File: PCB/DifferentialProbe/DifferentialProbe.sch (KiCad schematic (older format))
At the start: 33 parts, among them U1 IFNU411, U2 HFA3046BZ

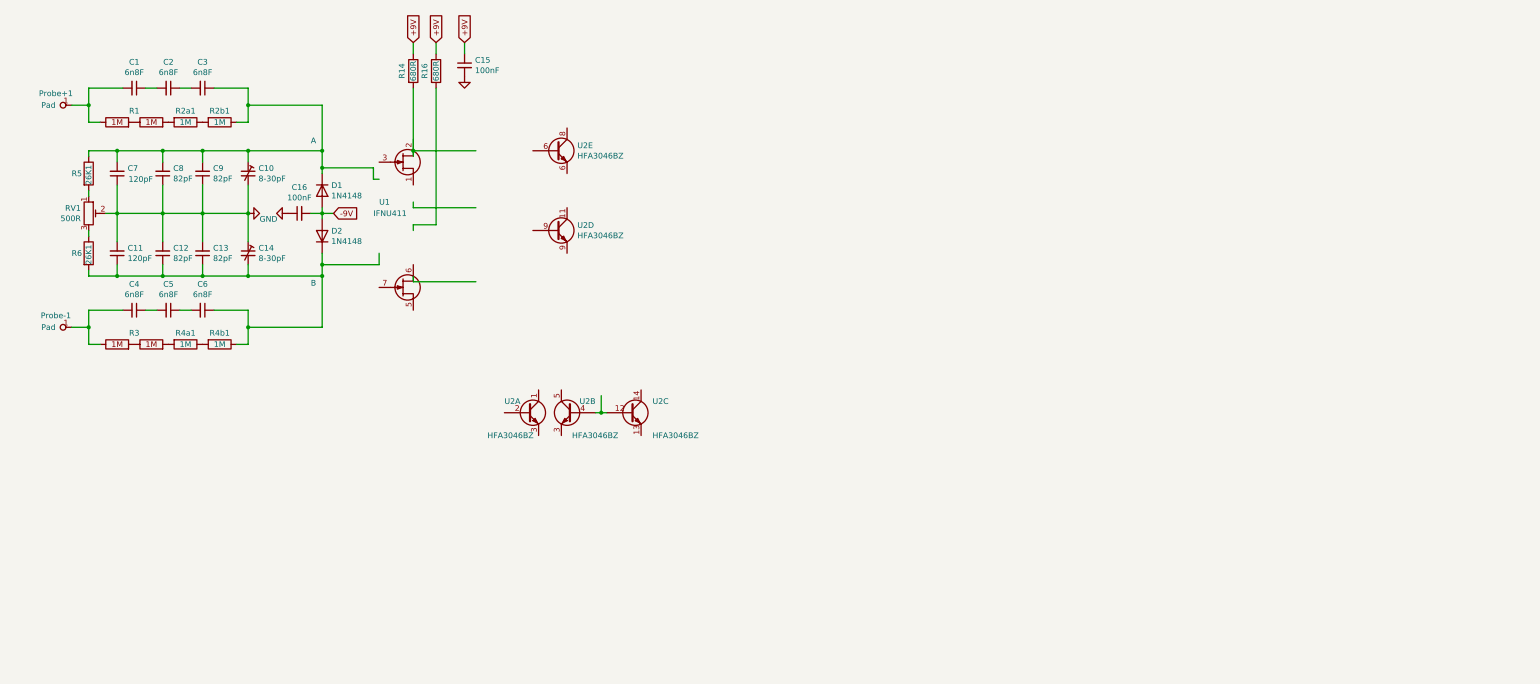
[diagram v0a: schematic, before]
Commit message: 1st design finished
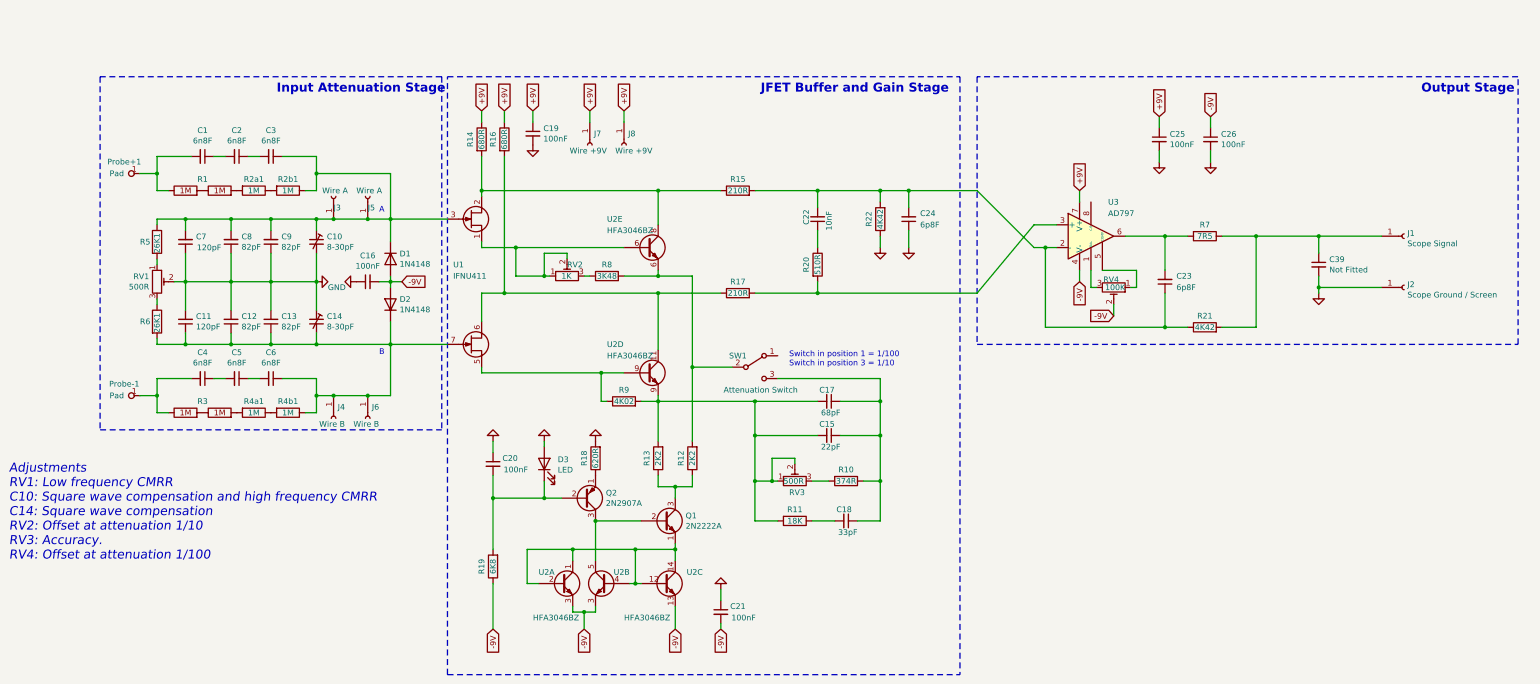
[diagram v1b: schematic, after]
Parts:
- added C15: 22pF, Capacitor_THT:C_Disc_D3.0mm_W1.6mm_P2.50mm, symbol Device:C_Small
- added C17: 68pF, Capacitor_THT:C_Disc_D3.0mm_W1.6mm_P2.50mm, symbol Device:C_Small
- added C18: 33pF, Capacitor_THT:C_Disc_D3.0mm_W1.6mm_P2.50mm, symbol Device:C_Small
- added C20, C21, C25, C26: 100nF, Capacitor_THT:C_Disc_D4.3mm_W1.9mm_P5.00mm, symbol Device:C_Small
- added C22: 10nF, Capacitor_THT:C_Disc_D3.0mm_W1.6mm_P2.50mm, symbol Device:C_Small
- added C23, C24: 6p8F, Capacitor_THT:C_Disc_D3.0mm_W1.6mm_P2.50mm, symbol Device:C_Small
- added C39: Not Fitted, Capacitor_THT:C_Disc_D4.3mm_W1.9mm_P5.00mm, symbol Device:C_Small
- added D3: LED, LED_THT:LED_D3.0mm, symbol Device:LED
- added J1: Scope Signal, Connector_Wire:SolderWire-2.5sqmm_1x01_D2.4mm_OD4.4mm, symbol Connector:Conn_01x01_Female
- added J2: Scope Ground / Screen, Connector_Wire:SolderWire-2.5sqmm_1x01_D2.4mm_OD4.4mm, symbol Connector:Conn_01x01_Female
- added J3, J5: Wire A, BVKSound:Wire_Hole, symbol BVKSound:Wire
- added J4, J6: Wire B, BVKSound:Wire_Hole, symbol BVKSound:Wire
- added J7, J8: Wire +9V, BVKSound:Wire_Hole, symbol BVKSound:Wire
- added Q1: 2N2222A, Package_TO_SOT_THT:TO-18-3, symbol Device:Q_NPN_EBC
- added Q2: 2N2907A, Package_TO_SOT_THT:TO-18-3, symbol Device:Q_PNP_EBC
- added R10: 374R, Resistor_THT:R_Axial_DIN0207_L6.3mm_D2.5mm_P10.16mm_Horizontal, symbol Device:R
- added R11: 18K, Resistor_THT:R_Axial_DIN0204_L3.6mm_D1.6mm_P7.62mm_Horizontal, symbol Device:R
- added R12, R13: 2K2, Resistor_THT:R_Axial_DIN0207_L6.3mm_D2.5mm_P10.16mm_Horizontal, symbol Device:R
- added R15: 210R, Resistor_THT:R_Axial_DIN0207_L6.3mm_D2.5mm_P10.16mm_Horizontal, symbol Device:R
- added R17: 210R, Resistor_THT:R_Axial_DIN0207_L6.3mm_D2.5mm_P2.54mm_Vertical, symbol Device:R
- added R18: 620R, Resistor_THT:R_Axial_DIN0207_L6.3mm_D2.5mm_P2.54mm_Vertical, symbol Device:R
- added R19: 6K8, Resistor_THT:R_Axial_DIN0207_L6.3mm_D2.5mm_P10.16mm_Horizontal, symbol Device:R
- added R20: 510R, Resistor_THT:R_Axial_DIN0204_L3.6mm_D1.6mm_P7.62mm_Horizontal, symbol Device:R
- added R21, R22: 4K42, Resistor_THT:R_Axial_DIN0207_L6.3mm_D2.5mm_P10.16mm_Horizontal, symbol Device:R
- added R7: 7R5, Resistor_THT:R_Axial_DIN0204_L3.6mm_D1.6mm_P7.62mm_Horizontal, symbol Device:R
- added R8: 3K48, Resistor_THT:R_Axial_DIN0207_L6.3mm_D2.5mm_P10.16mm_Horizontal, symbol Device:R
- added R9: 4K02, Resistor_THT:R_Axial_DIN0207_L6.3mm_D2.5mm_P10.16mm_Horizontal, symbol Device:R
- added RV2: 1K, BVKSound:67WR10KLF, symbol Device:R_POT_TRIM
- added RV3: 500R, BVKSound:3362P_1, symbol Device:R_POT_TRIM
- added RV4: 100K, BVKSound:64W_1, symbol Device:R_POT_TRIM
- added SW1: Attenuation Switch, BVKSound:SSSF011700, symbol Switch:SW_SPDT
- added U3: AD797, Package_DIP:DIP-8_W7.62mm, symbol Amplifier_Operational:AD797
- R16: footprint Resistor_THT:R_Axial_DIN0204_L3.6mm_D1.6mm_P2.54mm_Vertical -> Resistor_THT:R_Axial_DIN0207_L6.3mm_D2.5mm_P2.54mm_Vertical
- renumbered C15 to C19
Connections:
- wire segments 89 -> 215
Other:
- note added: "Adjustments\nRV1: Low frequency CMRR\nC10: Square wave compensation and high frequency CMRR\nC14: Square wave compensation\nRV2: Offset at attenuation 1/10\nRV3: Accuracy.\nRV4: Offset at attenuation 1/100"
- note added: "Input Attenuation Stage"
- note added: "JFET Buffer and Gain Stage"
- note added: "Output Stage"
- note added: "Switch in position 1 = 1/100\nSwitch in position 3 = 1/10"
- moved on the sheet: C1, C10, C11, C12, C13, C14, C16, C19, C2, C3, C4, C5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
